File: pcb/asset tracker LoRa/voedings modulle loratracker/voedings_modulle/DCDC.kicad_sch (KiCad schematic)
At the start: 0 parts

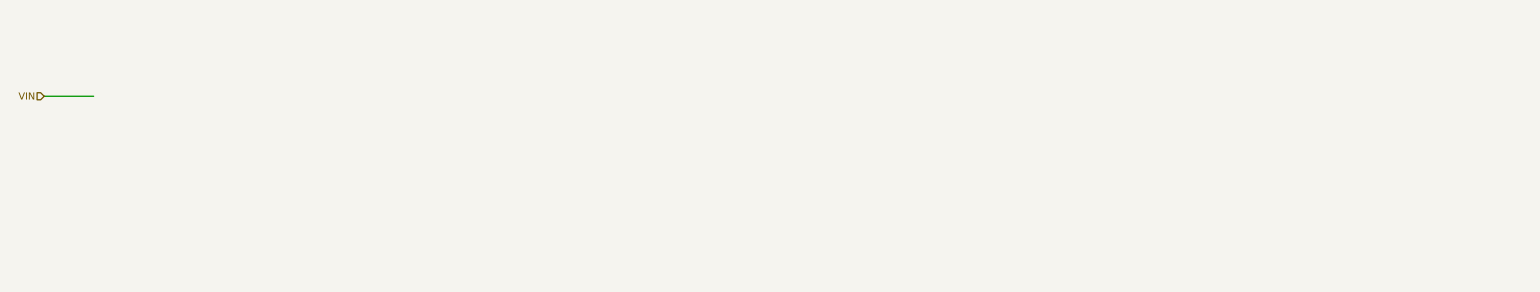
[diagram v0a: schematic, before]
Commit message: wef
wef
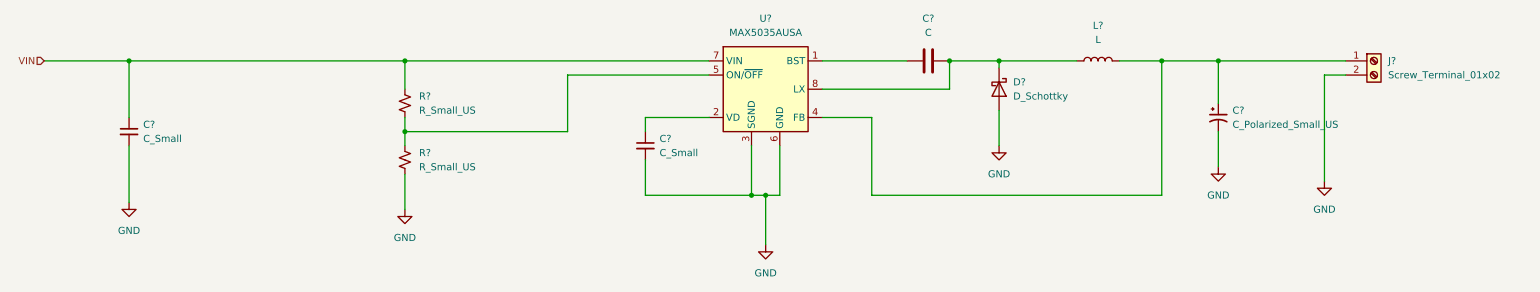
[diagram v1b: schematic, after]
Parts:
- added C?: C_Polarized_Small_US, symbol Device:C_Polarized_Small_US
- added C? (x2): C_Small, symbol Device:C_Small
- added C?: C, symbol Device:C
- added D?: D_Schottky, symbol Device:D_Schottky
- added J?: Screw_Terminal_01x02, symbol Connector:Screw_Terminal_01x02
- added L?: L, symbol Device:L
- added R? (x2): R_Small_US, symbol Device:R_Small_US
- added U?: MAX5035AUSA, Package_SO:SOIC-8_3.9x4.9mm_P1.27mm, symbol Regulator_Switching:MAX5035AUSA
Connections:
- net VIN: now also C?.1, R?.1, U?.7 (VIN)
- new net: R?.1, R?.2, U?.5 (ON/~{OFF})
- new net: C?.2, D?.1 (K), L?.1, U?.8 (LX)
- new net: C?.1, J?.1 (Pin_1), L?.2, U?.4 (FB)
- new net: C?.1, U?.1 (BST)
- new net: C?.1, U?.2 (VD)
- new net GND: C?.2, C?.2, C?.2, D?.2 (A), J?.2 (Pin_2), R?.2, U?.3 (SGND), U?.6 (GND)
